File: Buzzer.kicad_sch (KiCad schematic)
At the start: 5 parts, among them J1 BuzzConn, Q3 AO3400A

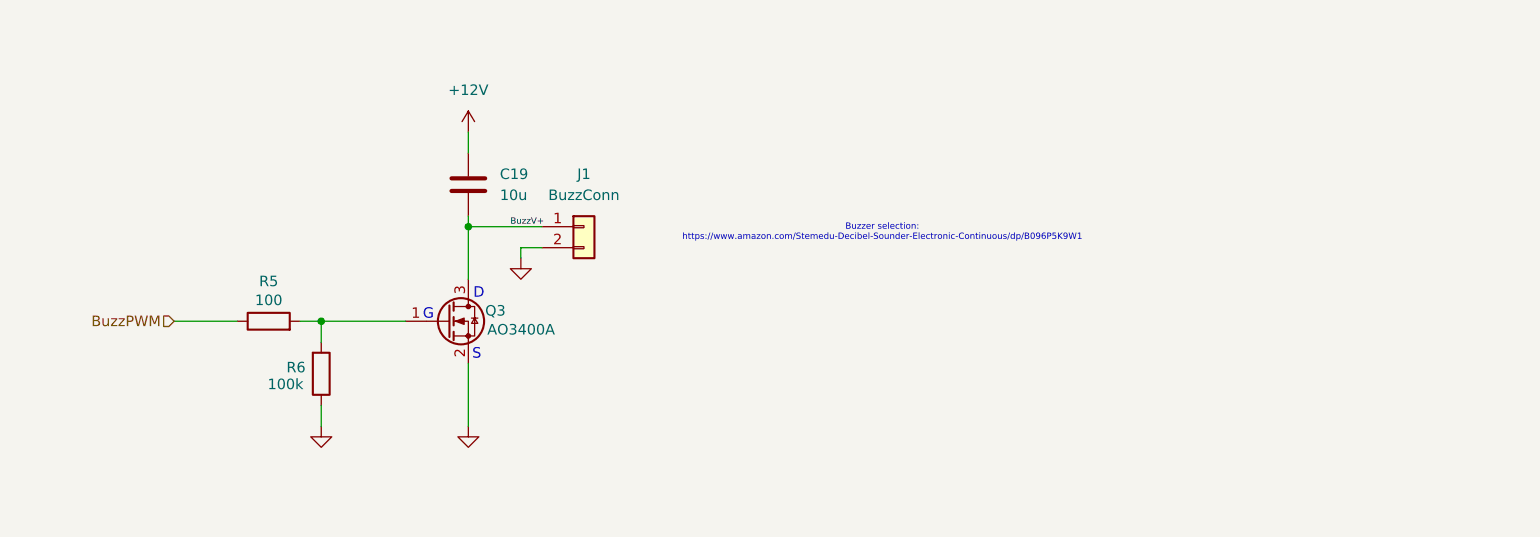
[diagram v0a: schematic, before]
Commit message: revA4
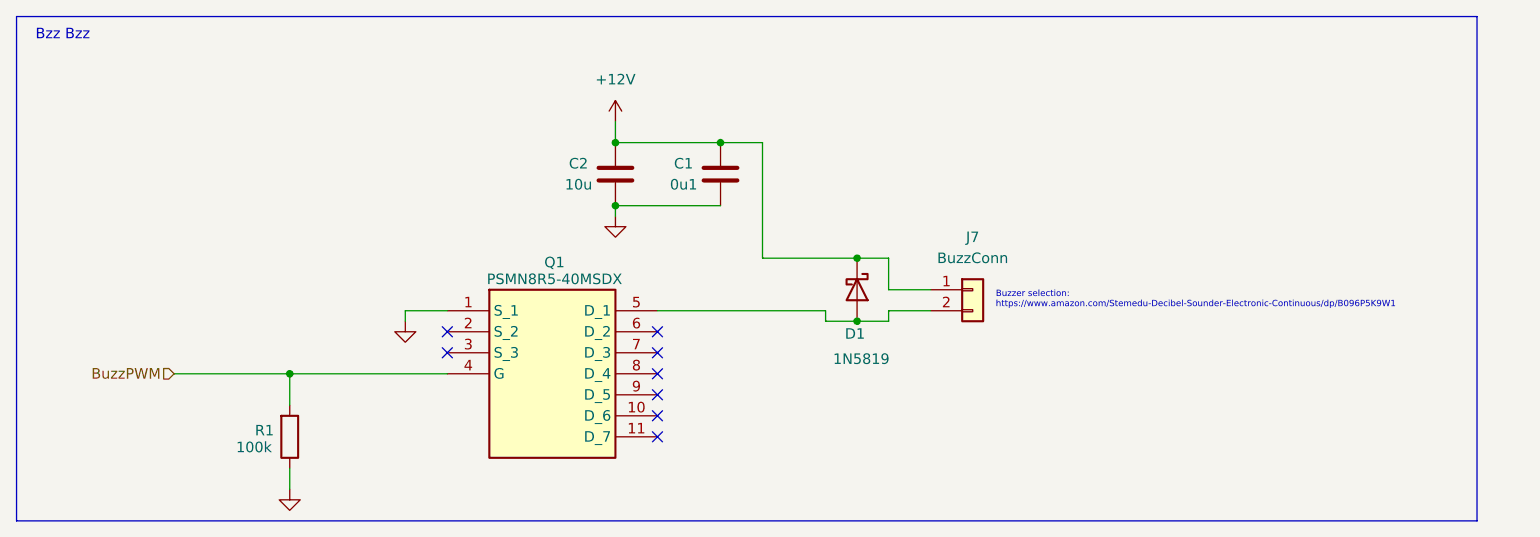
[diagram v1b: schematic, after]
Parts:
- removed C19: 10u, symbol Device:C
- removed J1: BuzzConn, symbol Connector_Generic:Conn_01x02
- removed Q3: AO3400A, Package_TO_SOT_SMD:SOT-23, symbol Transistor_FET:AO3400A
- removed R5: 100, symbol Device:R
- removed R6: 100k, symbol Device:R
- added C1: 0u1, symbol Device:C
- added C2: 10u, symbol Device:C
- added D1: 1N5819, Diode_THT:D_DO-41_SOD81_P10.16mm_Horizontal, symbol Diode:1N5819
- added J7: BuzzConn, symbol Connector_Generic:Conn_01x02
- added Q1: PSMN8R5-40MSDX, BUK7M1780EX, symbol utsvt_power:PSMN8R5-40MSDX
- added R1: 100k, symbol Device:R
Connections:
- net +12V: now also C1.1, C2.1, D1.1 (K), J7.1 (Pin_1)
- net BuzzPWM: now also Q1.4 (G), R1.2
- net GND: now also C1.2, C2.2, Q1.1 (S_1), R1.1
- new net: D1.2 (A), J7.2 (Pin_2), Q1.5 (D_1)
- no-connect marks 0 -> 8
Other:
- note added: "Bzz Bzz"
- note removed: "D"
- note removed: "G"
- note removed: "S"

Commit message: RevA5
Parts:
- C1: footprint (none) -> Capacitor_SMD:C_0603_1608Metric
- C2: footprint (none) -> Capacitor_SMD:C_0805_2012Metric
- R1: footprint (none) -> Resistor_SMD:R_0603_1608Metric
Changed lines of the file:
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@@
 			)
 		)
-		(property "Footprint" ""
+		(property "Footprint" "Resistor_SMD:R_0603_1608Metric"
 			(at 51.562 67.31 90)
 			(effects
@@
 			)
 		)
-		(property "Footprint" ""
+		(property "Footprint" "Capacitor_SMD:C_0805_2012Metric"
 			(at 91.7448 39.37 0)
 			(effects
@@
 			)
 		)
-		(property "Footprint" ""
+		(property "Footprint" "Capacitor_SMD:C_0603_1608Metric"
 			(at 104.4448 39.37 0)
 			(effects

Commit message: RevA6
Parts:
- J7: footprint (none) -> 1053091202
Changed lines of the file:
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@@
 			)
 		)
-		(property "Footprint" ""
+		(property "Footprint" "1053091202"
 			(at 135.89 49.53 0)
 			(effects
@@
 			)
 		)
-		(property "Datasheet" "https://www.amazon.com/Stemedu-Decibel-Sounder-Electronic-Continuous/dp/B096P5K9W1"
+		(property "Datasheet" "https://www.molex.com/en-us/products/part-detail/1053091202?display=pdf"
 			(at 135.89 49.53 0)
 			(effects

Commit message: RevA6 footprint updates
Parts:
- J7: footprint 1053091202 -> 153091202:1053091202
- Q1: footprint BUK7M1780EX -> UTSVT_Power:PSMN8R5-40MSDX
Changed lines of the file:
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@@
 			)
 		)
-		(property "Footprint" "1053091202"
+		(property "Footprint" "153091202:1053091202"
 			(at 135.89 49.53 0)
 			(effects
@@
 			)
 		)
-		(property "Footprint" "BUK7M1780EX"
+		(property "Footprint" "UTSVT_Power:PSMN8R5-40MSDX"
 			(at 93.98 146.99 0)
 			(effects
